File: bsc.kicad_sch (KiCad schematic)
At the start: 62 parts, among them J1 AVR-ISP-6, J11 Conn_02x05_Odd_Even, J2 Prog, J3 U0TXD silent, J4 Boot, K1 TIANBO-HJR-4102-L, Q1 BSS138, U1 LMO78_03-0.5, U2 ESP32WROOM32E16, U3 ATtiny24A-SS, U4 ADuM1201AR, U5 ADuM1201AR, U6 ADuM1201AR, U7 SN65HVD234, U8 SP3485EN, U9 SP3485EN, X1 Conn_S2, X2 Conn_S1, X4 Conn_SV

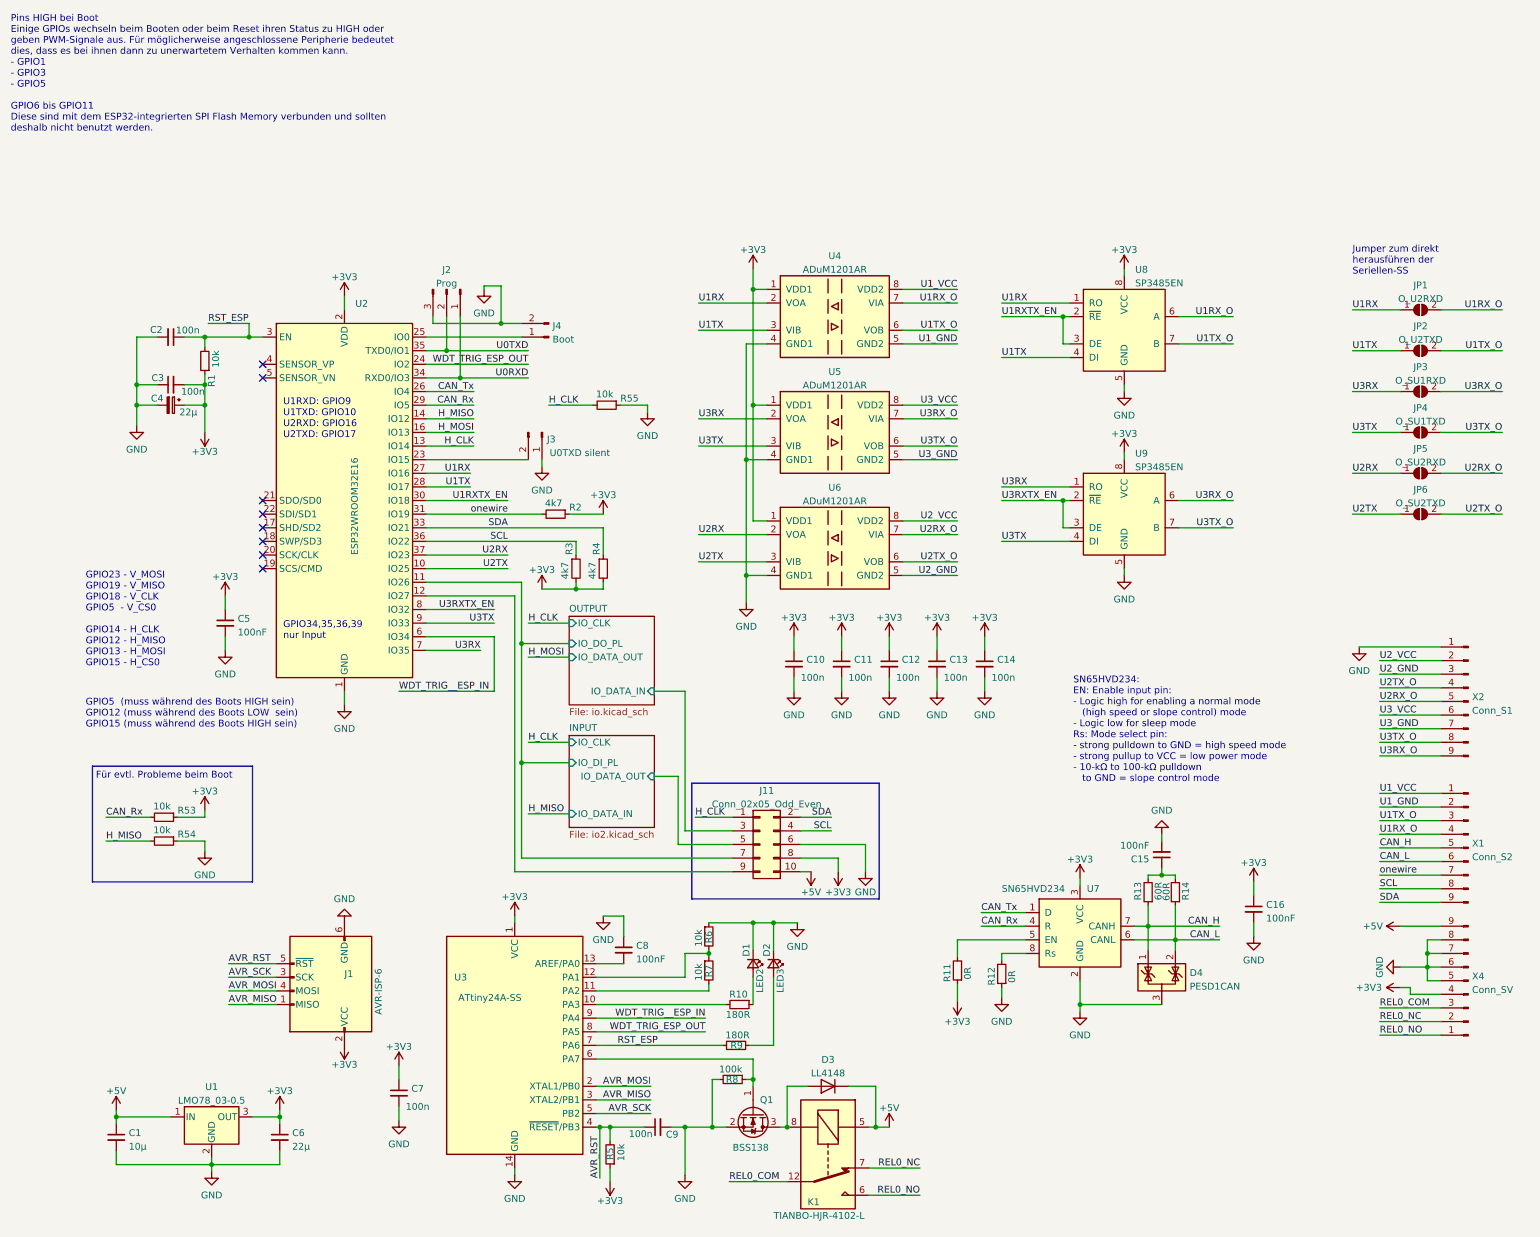
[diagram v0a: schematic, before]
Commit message: Redesign PCB
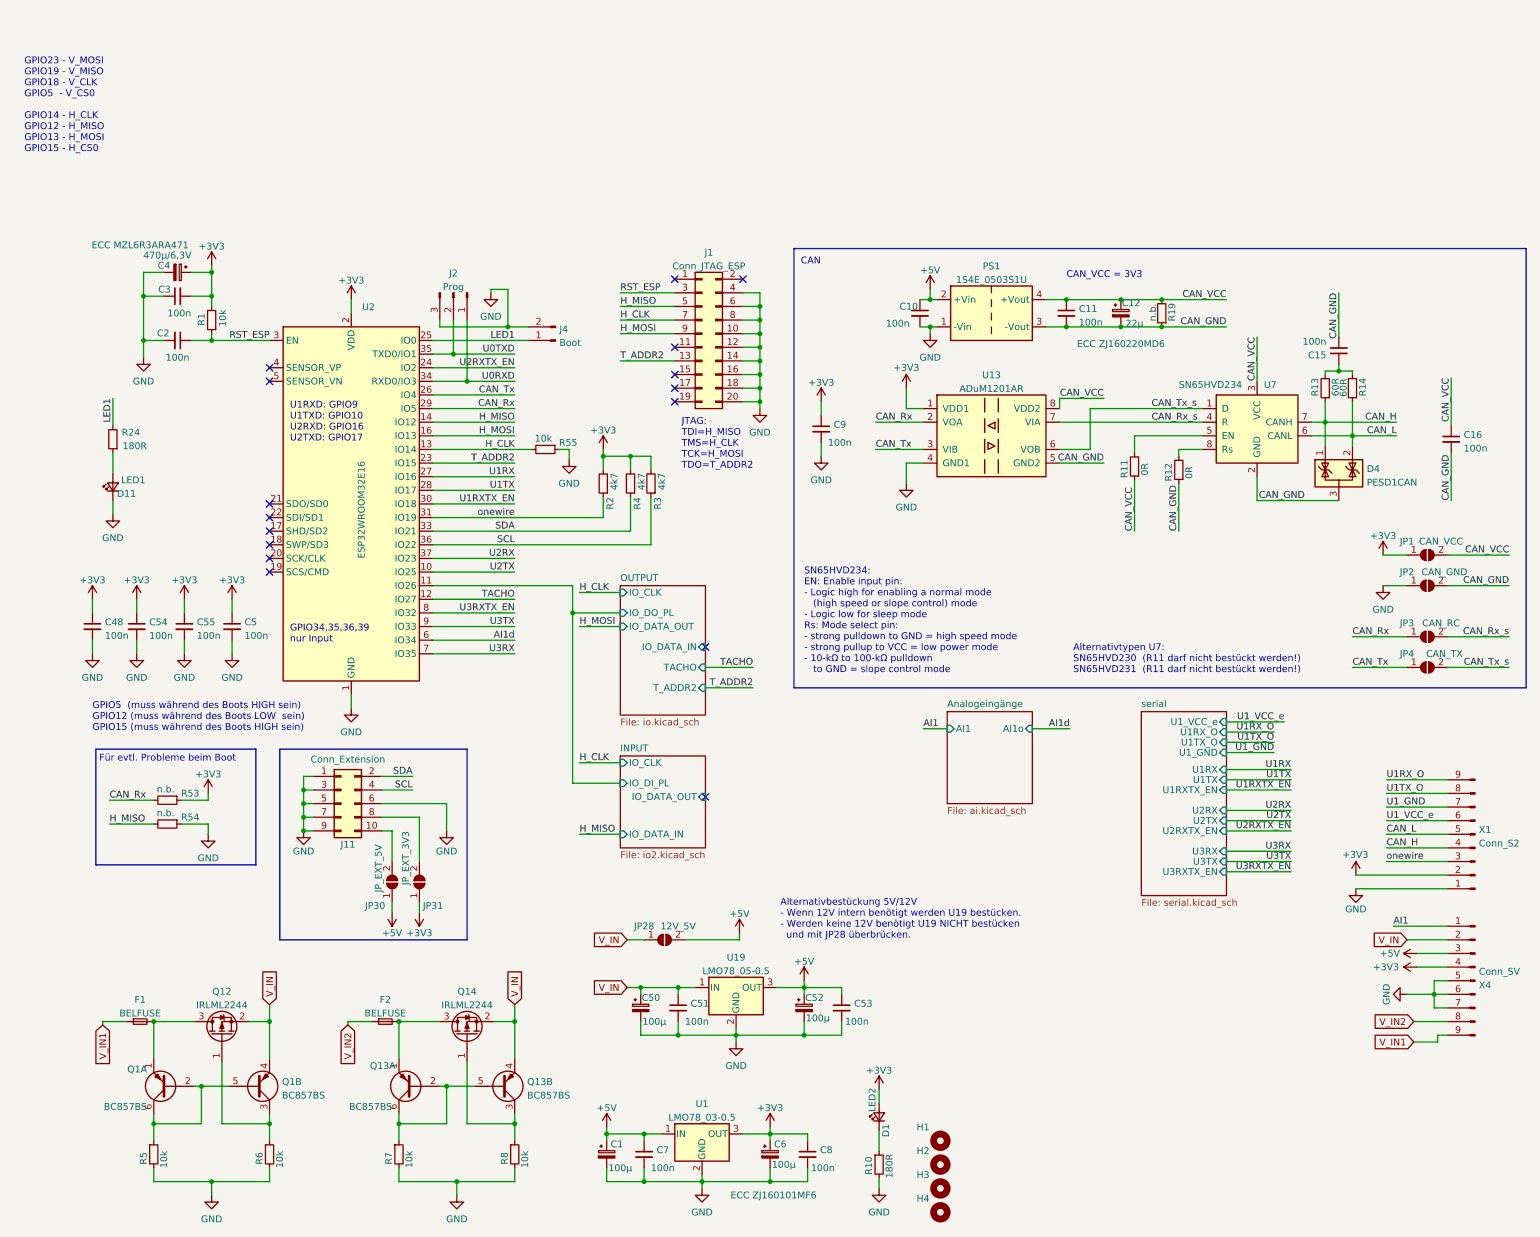
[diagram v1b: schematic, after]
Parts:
- removed C1: 10µ, Capacitor_SMD:CP_Elec_6.3x5.9, symbol Device:C_Small
- removed C12, C13, C14: 100n, Capacitor_SMD:C_0603_1608Metric, symbol Device:C_Small
- removed C6: 22µ, Capacitor_SMD:CP_Elec_6.3x5.9, symbol Device:C_Small
- removed D2: LED3, LED_SMD:LED_PLCC-2, symbol Device:LED_Small
- removed D3: LL4148, Diode_SMD:D_MiniMELF, symbol Diode:LL4148
- removed J1: AVR-ISP-6, Connector_PinHeader_2.54mm:PinHeader_2x03_P2.54mm_Vertical, symbol Connector:AVR-ISP-6
- removed J3: U0TXD silent, Connector_PinHeader_2.54mm:PinHeader_1x02_P2.54mm_Vertical, symbol Connector:Conn_01x02_Male
- removed JP5: O_SU2RXD, Jumper:SolderJumper-2_P1.3mm_Open_RoundedPad1.0x1.5mm, symbol Jumper:SolderJumper_2_Open
- removed JP6: O_SU2TXD, Jumper:SolderJumper-2_P1.3mm_Open_RoundedPad1.0x1.5mm, symbol Jumper:SolderJumper_2_Open
- removed K1: TIANBO-HJR-4102-L, Relay_THT:Relay_SPDT_HJR-4102, symbol Relay:TIANBO-HJR-4102-L
- removed Q1: BSS138, Package_TO_SOT_SMD:SOT-23, symbol Transistor_FET:BSS138
- removed R9: 180R, Resistor_SMD:R_0603_1608Metric, symbol Device:R_Small
- removed U3: ATtiny24A-SS, Package_SO:SOIC-14_3.9x8.7mm_P1.27mm, symbol MCU_Microchip_ATtiny:ATtiny24A-SS
- removed U4, U5, U6: ADuM1201AR, Package_SO:SOIC-8_3.9x4.9mm_P1.27mm, symbol Isolator:ADuM1201AR
- removed U8, U9: SP3485EN, Package_SO:SOIC-8_3.9x4.9mm_P1.27mm, symbol Interface_UART:SP3485EN
- removed X2: Conn_S1, Connector_Phoenix_MC:PhoenixContact_MCV_1,5_9-G-3.81_1x09_P3.81mm_Vertical, symbol Connector:Conn_01x09_Male
- added C1, C50, C52, C6: 100µ, Capacitor_SMD:CP_Elec_6.3x5.9, symbol Device:C_Polarized_Small
- added C12: 22µ, Capacitor_SMD:CP_Elec_4x5.8, symbol Device:C_Polarized_Small
- added C48, C51, C53, C54, C55: 100n, Capacitor_SMD:C_0603_1608Metric, symbol Device:C_Small
- added D11: LED1, LED_SMD:LED_PLCC-2, symbol Device:LED_Small
- added F1, F2: BELFUSE, Fuse:Fuse_0679H, symbol Device:Fuse_Small
- added H1, H2, H3, H4: MountingHole, MountingHole:MountingHole_3.2mm_M3, symbol Mechanical:MountingHole
- added J1: Conn_JTAG_ESP, Connector_PinHeader_1.27mm:PinHeader_2x10_P1.27mm_Vertical_SMD, symbol Connector_Generic:Conn_02x10_Odd_Even
- added JP28: 12V_5V, Jumper:SolderJumper-2_P1.3mm_Open_RoundedPad1.0x1.5mm, symbol Jumper:SolderJumper_2_Open
- added JP30: JP_EXT_5V, Jumper:SolderJumper-2_P1.3mm_Open_RoundedPad1.0x1.5mm, symbol Jumper:SolderJumper_2_Open
- added JP31: JP_EXT_3V3, Jumper:SolderJumper-2_P1.3mm_Open_RoundedPad1.0x1.5mm, symbol Jumper:SolderJumper_2_Open
- added PS1: 1S4E_0503S1U, custom_th:Converter_DCDC_GAPTEC_1S4E_S1U, symbol Converter_DCDC:MEE1S0303SC
- added Q1, Q13: BC857BS, Package_TO_SOT_SMD:SOT-363_SC-70-6, symbol Transistor_BJT:BC857BS
- added Q12, Q14: IRLML2244, Package_TO_SOT_SMD:SOT-23, symbol Transistor_FET:IRLML5203
- added R19: n.b., Resistor_SMD:R_0603_1608Metric, symbol Device:R_Small
- added R24: 180R, Resistor_SMD:R_0603_1608Metric, symbol Device:R_Small
- added U13: ADuM1201AR, Package_SO:SOIC-8_3.9x4.9mm_P1.27mm, symbol Isolator:ADuM1201AR
- added U19: LMO78_05-0.5, custom_th:Converter_DCDC_RECOM_R-78E-1.0, symbol Regulator_Switching:R-78E3.3-0.5
- C15, C16, C5, C8: value 100nF -> 100n
- C4: value 22µ -> 470µ/6,3V; footprint Capacitor_SMD:CP_Elec_6.3x5.9 -> Capacitor_SMD:CP_Elec_8x10; Reichelt (none) -> ECC MZL6R3ARA471
- J11: value Conn_02x05_Odd_Even -> Conn_Extension; footprint Connector_PinSocket_2.54mm:PinSocket_2x05_P2.54mm_Vertical -> Connector_PinHeader_2.54mm:PinHeader_2x05_P2.54mm_Vertical
- JP1: value O_U2RXD -> CAN_VCC
- JP2: value O_U2TXD -> CAN_GND
- JP3: value O_SU1RXD -> CAN_RC
- JP4: value O_SU1TXD -> CAN_TX
- R53, R54: value 10k -> n.b.
- R8: value 100k -> 10k
- U1: footprint Converter_DCDC:Converter_DCDC_RECOM_R-78E-0.5_THT -> custom_th:Converter_DCDC_RECOM_R-78E-1.0
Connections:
- net REL0_COM is gone; now on net +5V: X4.3 (Pin_3)
- net U1_VCC is gone; now on net GND: X1.1 (Pin_1)
- net +3V3: now also C8.1, C9.1, D1.2 (A), JP1.1 (A), R1.2, R2.2, X1.2 (Pin_2), C48.1, C54.1, C55.1, C6.1, JP31.1 (A), U13.1 (VDD1); no longer C10.1, C11.1, C16.1, C7.1, J11.8 (Pin_8), R1.1, R11.1, R2.1, R5.1, U7.3 (VCC)
- net +5V: now also C10.1, C7.1, C1.1, C52.1, C53.1, JP28.2 (B), JP30.1 (A), PS1.2 (+Vin), U19.3 (OUT); no longer J11.10 (Pin_10), X4.9 (Pin_9)
- net CAN_H: now also X1.4 (Pin_4); no longer X1.5 (Pin_5)
- net CAN_L: now also X1.5 (Pin_5); no longer X1.6 (Pin_6)
- net CAN_Rx: now also JP3.1 (A), U13.2 (VOA); no longer U7.4 (R)
- net CAN_Tx: now also JP4.1 (A), U13.3 (VIB); no longer U7.1 (D)
- net GND: now also C8.2, J11.1 (Pin_1), J11.3 (Pin_3), J11.5 (Pin_5), J11.7 (Pin_7), J11.9 (Pin_9), JP2.1 (A), R10.2, R5.2, R6.2, R7.2, C1.2, C48.2, C50.2, C51.2, C52.2, C53.2, C54.2, C55.2, C6.2, D11.1 (K), J1.10 (Pin_10), J1.12 (Pin_12), J1.14 (Pin_14), J1.16 (Pin_16), J1.18 (Pin_18), J1.20 (Pin_20), J1.4 (Pin_4), J1.6 (Pin_6), J1.8 (Pin_8), PS1.1 (-Vin), U13.4 (GND1), U19.2 (GND); no longer C11.2, C15.2, C16.2, C8.1, D1.1 (K), D4.3 (A), R12.1, R6.1, U7.2 (GND), X4.8 (Pin_8)
- net H_CLK: now also J1.7 (Pin_7); no longer J11.1 (Pin_1)
- net H_MISO: now also J1.5 (Pin_5)
- net H_MOSI: now also J1.9 (Pin_9)
- net INPUT/IO_DATA_OUT: no longer J11.5 (Pin_5)
- net INPUT/IO_DI_PL: no longer J11.7 (Pin_7)
- net OUTPUT/IO_DATA_IN: no longer J11.3 (Pin_3)
- net RST_ESP: now also R1.1, J1.3 (Pin_3); no longer R1.2
- net SCL: no longer X1.8 (Pin_8)
- net SDA: no longer X1.9 (Pin_9)
- net U1RX: no longer JP1.1 (A)
- net U1RX_O: now also X1.9 (Pin_9); no longer JP1.2 (B), X1.4 (Pin_4)
- net U1TX: no longer JP2.1 (A)
- net U1TX_O: now also X1.8 (Pin_8); no longer JP2.2 (B), X1.3 (Pin_3)
- net U1_GND: now also X1.7 (Pin_7); no longer X1.2 (Pin_2)
- net U3RX: no longer JP3.1 (A)
- net U3TX: no longer JP4.1 (A)
- net onewire: now also R2.1, X1.3 (Pin_3); no longer R2.2, X1.7 (Pin_7)
- net at R8.1: now also Q13.3 (C2), Q14.1 (G)
- net at R7.1: now also Q13.2 (B1), Q13.5 (B2), Q13.6 (C1); no longer R6.2
- net at R10.1: now also D1.1 (K); no longer D1.2 (A)
- net TACHO: now reaches U2.12 (IO27)
- net TACHO: no longer J11.9 (Pin_9)
- net T_ADDR2: now reaches U2.23 (IO15)
- net T_ADDR2: now also J1.13 (Pin_13)
- net LED1: now reaches J4.1 (Pin_1), U2.25 (IO0)
- net LED1: now also R24.2
- removed net AVR_RST: C9.1, R5.2
- net REL0_NC renamed V_IN
- net V_IN: now also C50.1, C51.1, JP28.1 (A), Q1.4 (E2), Q12.2 (S), Q13.4 (E2), Q14.2 (S), U19.1 (IN)
- net REL0_NO renamed AI1
- net U3RX_O renamed CAN_Rx_s
- net CAN_Rx_s: now also U7.4 (R), U13.7 (VIA)
- net U3TX_O renamed CAN_Tx_s
- net CAN_Tx_s: now also U7.1 (D), U13.6 (VOB)
- net WDT_TRIG_ESP_OUT renamed U2RXTX_EN
- net WDT_TRIG__ESP_IN renamed AI1d
- new net: J11.10 (Pin_10), JP30.2 (B)
- new net: F2.2, Q13.1 (E1), Q14.3 (D)
- new net: Q1.3 (C2), Q12.1 (G), R6.1
- new net: Q1.2 (B1), Q1.5 (B2), Q1.6 (C1), R5.1
- new net: F1.2, Q1.1 (E1), Q12.3 (D)
- new net: D11.2 (A), R24.1
- new net: J11.8 (Pin_8), JP31.2 (B)
- new net CAN_GND: C11.2, C12.2, C15.2, C16.2, D4.3 (A), JP2.2 (B), PS1.3 (-Vout), R12.1, R19.1, U13.5 (GND2), U7.2 (GND)
- new net CAN_VCC: C11.1, C12.1, C16.1, JP1.2 (B), PS1.4 (+Vout), R11.1, R19.2, U13.8 (VDD2), U7.3 (VCC)
- new net U1_VCC_e: X1.6 (Pin_6)
- new net V_IN1: F1.1, X4.9 (Pin_9)
- new net V_IN2: F2.1, X4.8 (Pin_8)
- no-connect marks 8 -> 16
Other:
- added sheet Analogeingänge (ai.kicad_sch)
- added sheet serial (serial.kicad_sch)
- sheet OUTPUT ports: added TACHO, T_ADDR2; removed none
- note added: "Alternativbestückung 5V/12V - Wenn 12V intern benötigt werden U19 bestücken. - Werden keine 12V benötigt U19 NICHT bestücken und mit JP28 überbrücken."
- note added: "Alternativtypen U7: SN65HVD230 (R11 darf nicht bestückt werden!) SN65HVD231 (R11 darf nicht bestückt werden!)"
- note added: "CAN"
- note added: "CAN_VCC = 3V3"
- note added: "JTAG: TDI=H_MISO TMS=H_CLK TCK=H_MOSI TDO=T_ADDR2"
- note removed: "Jumper zum direkt herausführen der Seriellen-SS"
- note removed: "Pins HIGH bei Boot Einige GPIOs wechseln beim Booten oder beim Reset ihren Status zu HIGH oder geben PWM-Signale aus. Für möglicherweise angeschlossene Peripherie bedeutet dies, dass es bei ihnen dann zu unerwartetem Verhalten kommen kann. - GPIO1 - GPIO3 - GPIO5 GPIO6 bis GPIO11 Diese sind mit dem ESP32-integrierten SPI Flash Memory verbunden und sollten deshalb nicht benutzt werden."
- moved on the sheet: C16, C2, C3, C4, C5, D1, D4, J11, J2, J4, R1, R10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
